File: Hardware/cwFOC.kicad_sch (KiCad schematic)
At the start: 6 parts

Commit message: 基本完成PCB设计
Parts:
- H1, H2, H3, H4, H5, H6: footprint MountingHole:MountingHole_2.2mm_M2_Pad_TopBottom -> myLib:MountingHole_2.2mm_M2
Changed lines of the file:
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@@
       (effects (font (size 1.27 1.27)) (justify left))
     )
-    (property "Footprint" "MountingHole:MountingHole_2.2mm_M2_Pad_TopBottom" (at 199.39 74.93 0)
+    (property "Footprint" "myLib:MountingHole_2.2mm_M2" (at 199.39 74.93 0)
       (effects (font (size 1.27 1.27)) hide)
     )
@@
       (effects (font (size 1.27 1.27)) (justify left))
     )
-    (property "Footprint" "MountingHole:MountingHole_2.2mm_M2_Pad_TopBottom" (at 199.39 85.09 0)
+    (property "Footprint" "myLib:MountingHole_2.2mm_M2" (at 199.39 85.09 0)
       (effects (font (size 1.27 1.27)) hide)
     )
@@
       (effects (font (size 1.27 1.27)) (justify left))
     )
-    (property "Footprint" "MountingHole:MountingHole_2.2mm_M2_Pad_TopBottom" (at 199.39 80.01 0)
+    (property "Footprint" "myLib:MountingHole_2.2mm_M2" (at 199.39 80.01 0)
       (effects (font (size 1.27 1.27)) hide)
     )
@@
       (effects (font (size 1.27 1.27)) (justify left))
     )
-    (property "Footprint" "MountingHole:MountingHole_2.2mm_M2_Pad_TopBottom" (at 199.39 100.33 0)
+    (property "Footprint" "myLib:MountingHole_2.2mm_M2" (at 199.39 100.33 0)
       (effects (font (size 1.27 1.27)) hide)
     )
@@
       (effects (font (size 1.27 1.27)) (justify left))
     )
-    (property "Footprint" "MountingHole:MountingHole_2.2mm_M2_Pad_TopBottom" (at 199.39 95.25 0)
+    (property "Footprint" "myLib:MountingHole_2.2mm_M2" (at 199.39 95.25 0)
       (effects (font (size 1.27 1.27)) hide)
     )
@@
       (effects (font (size 1.27 1.27)) (justify left))
     )
-    (property "Footprint" "MountingHole:MountingHole_2.2mm_M2_Pad_TopBottom" (at 199.39 90.17 0)
-      (effects (font (size 1.27 1.27)) hide)
-    )
+    (property "Footprint" "myLib:MountingHole_2.2mm_M2" (at 199.39 90.17 0)
+      (effects (font (size 1.27 1.27)) hide)
+    )

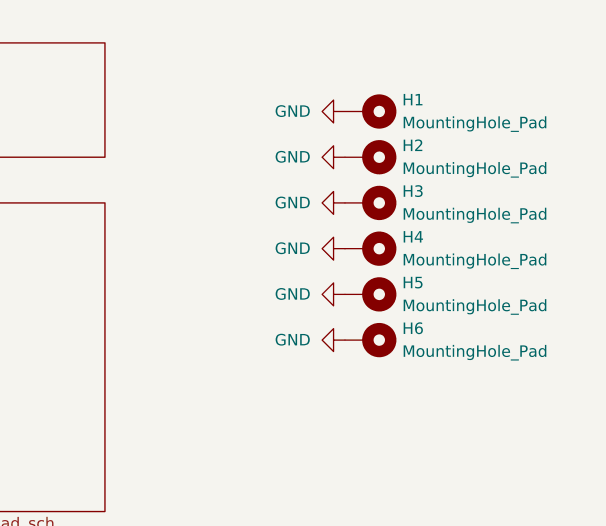
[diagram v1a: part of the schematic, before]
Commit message: 第一版硬件做好啦！(●'◡'●)
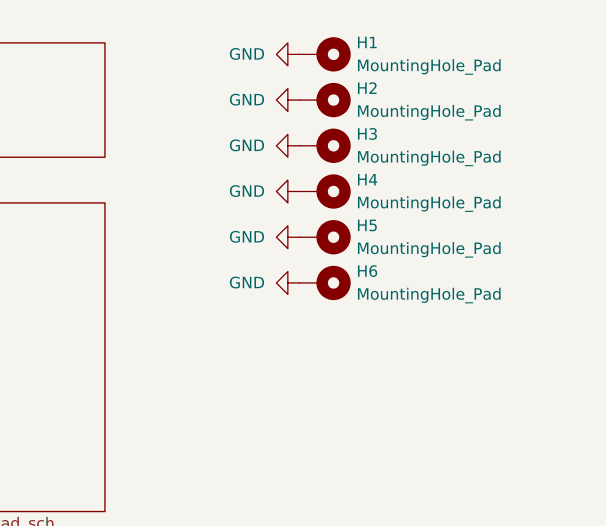
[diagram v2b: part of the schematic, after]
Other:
- company: akako -> Akako Industry
- title: mmFOC -> cwFOC
- moved on the sheet: H1, H2, H3, H4, H5, H6
